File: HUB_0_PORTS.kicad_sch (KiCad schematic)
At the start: 29 parts, among them U3 VL162, U8 TPS2560DRCR, U9 TPS2553DRVR-1

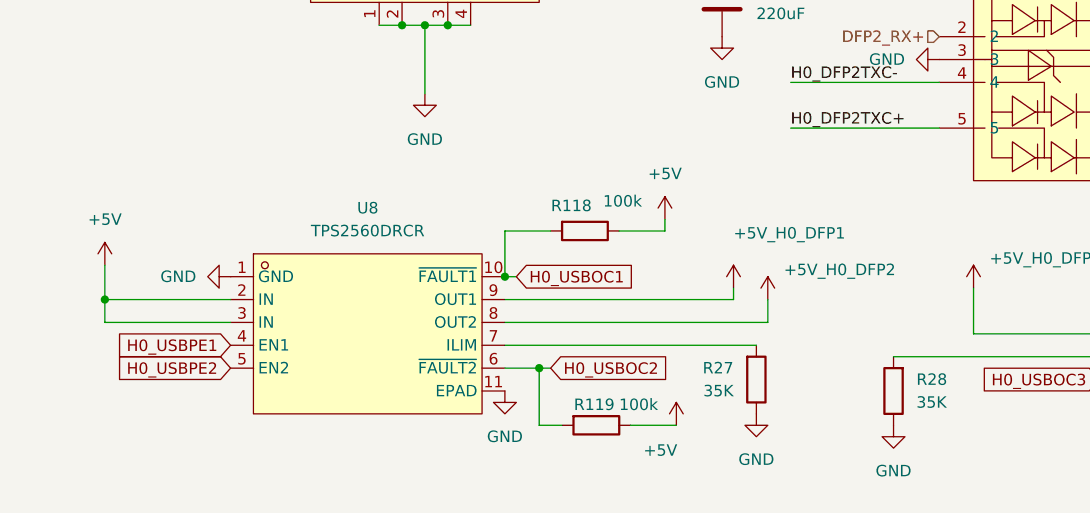
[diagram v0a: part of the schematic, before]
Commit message: .
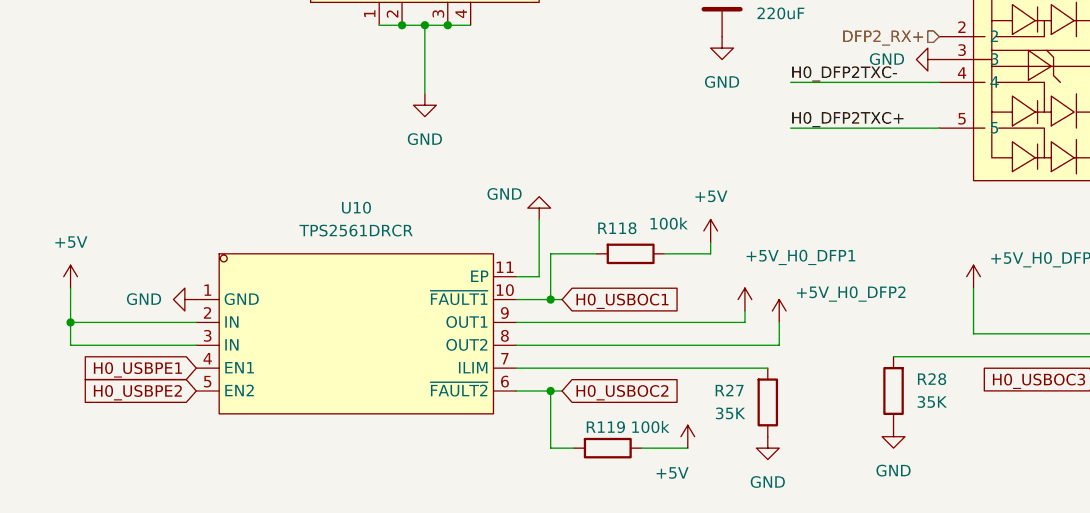
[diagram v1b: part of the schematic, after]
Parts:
- removed U8: TPS2560DRCR, easyeda2kicad:VSON-10_L3.0-W3.0-P0.50-BL-EP_TPS62410DRCR, symbol da:TPS2560DRCR
- added U10: TPS2561DRCR, easyeda2kicad:VSON-10_L3.0-W3.0-P0.50-TL-EP_TPS62410DRCR, symbol da:TPS2561DRCR
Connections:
- net +5V: now also U10.2 (IN), U10.3 (IN)
- net +5V_H0_DFP1: now also U10.9 (OUT1)
- net +5V_H0_DFP2: now also U10.8 (OUT2)
- net GND: now also U10.1 (GND), U10.11 (EP)
- net H0_USBOC1: now also U10.10 (~{FAULT1})
- net H0_USBOC2: now also U10.6 (~{FAULT2})
- net H0_USBPE1: now also U10.4 (EN1)
- net H0_USBPE2: now also U10.5 (EN2)
- net at R27.2: now also U10.7 (ILIM)
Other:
- moved on the sheet: R118, R119, R27
